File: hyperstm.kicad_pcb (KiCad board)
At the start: 2 copper layers, 71.5 x 70.1 mm, 28 parts, among them J1 USB_B_Micro, J10 SPI1, J2 DBG_HEADER, J3 Micro_SD_Card_Det, J4 Analog_Header, J5 UART_COMBO, J6 USART1, J7 SPI2, J8 I2C1, J9 I2C4, Q3 FDN340P, SW1 SW_SPST, SW2 SW_SPST, U1 STM32L4R5VITx, U2 MIC5219-3.3, U3 S27KL0641

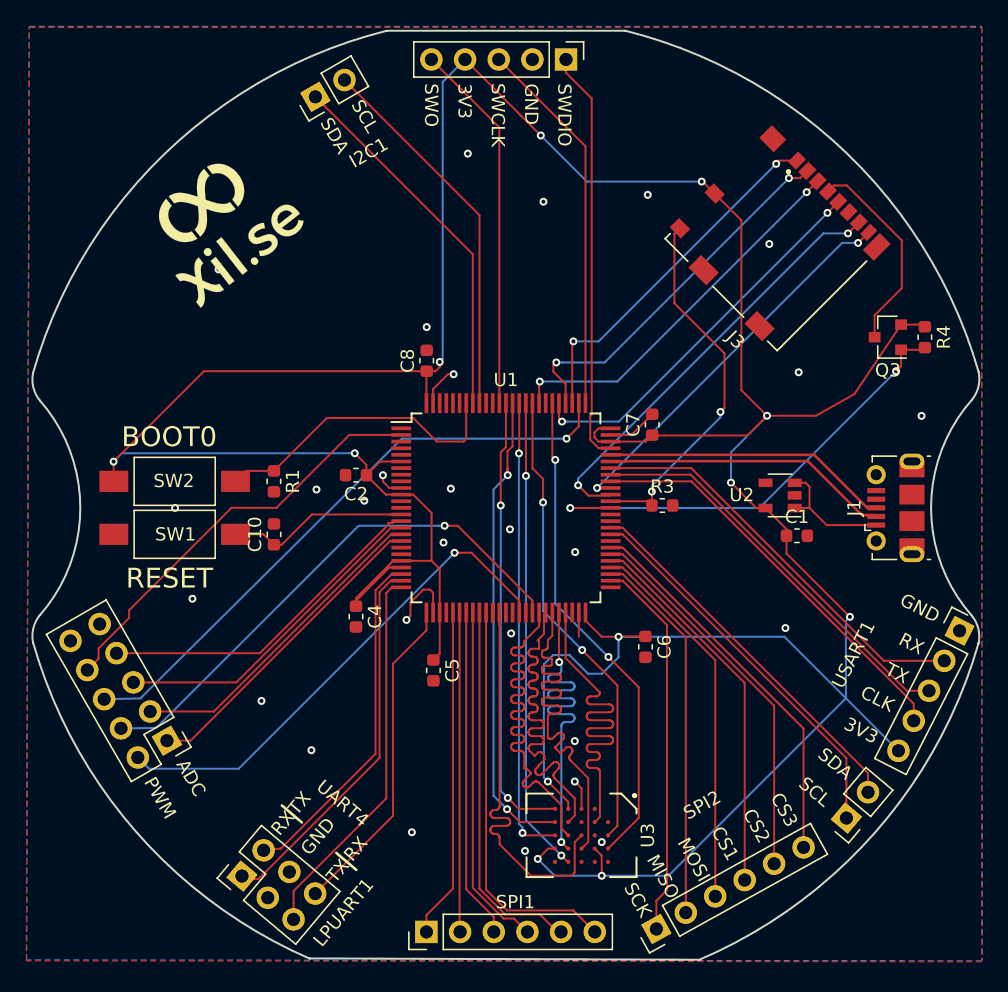
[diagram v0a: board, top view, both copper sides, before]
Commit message: Fix outline
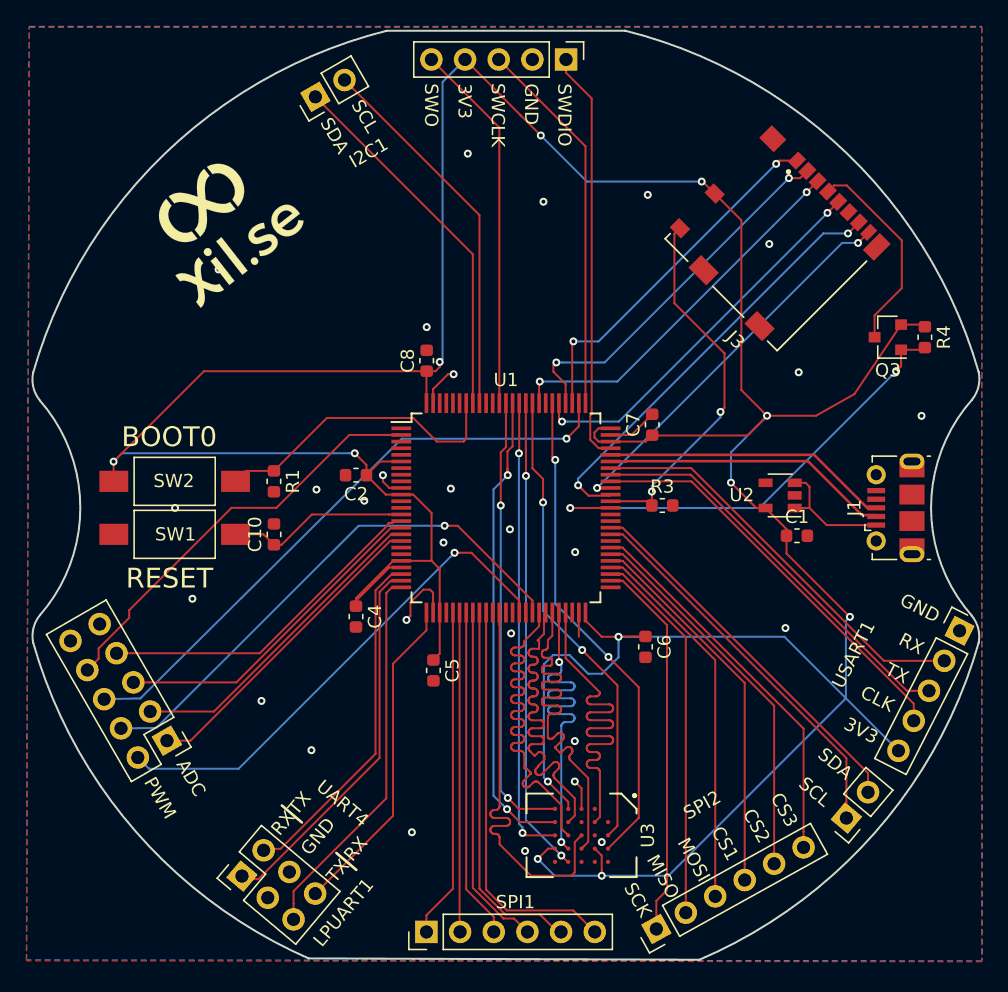
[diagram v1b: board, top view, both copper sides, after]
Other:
- outline, holes or cut-outs redrawn
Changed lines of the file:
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@@
-(kicad_pcb (version 20171130) (host pcbnew 5.0.0-fee4fd1~66~ubuntu18.04.1)
+(kicad_pcb (version 20171130) (host pcbnew 5.1.5+dfsg1-2build2)
   (general
     (thickness 1.6)
@@
     (zone_45_only no)
     (trace_min 0.1524)
-    (segment_width 0.2)
-    (edge_width 0.15)
     (via_size 0.6)
     (via_drill 0.3)
@@
     (uvia_min_size 0.2)
     (uvia_min_drill 0.1)
+    (edge_width 0.15)
+    (segment_width 0.2)
     (pcb_text_width 0.3)
     (pcb_text_size 1.5 1.5)
@@
       (xy 0.186687 3.496485) (xy 0.239391 3.49077) (xy 0.268318 3.491476)) (layer F.SilkS) (width 0.01))
   )
+  (gr_arc (start 183.24 109.71) (end 185.667211 110.189202) (angle -50.74504922) (layer Edge.Cuts) (width 0.15))
+  (gr_arc (start 150.01 100.02) (end 114.322718 110.169442) (angle -50.44715247) (layer Edge.Cuts) (width 0.15))
+  (gr_arc (start 116.75 90.32) (end 114.325521 89.785729) (angle -52.22555031) (layer Edge.Cuts) (width 0.15))
+  (gr_arc (start 116.76 109.67) (end 114.830001 108.100001) (angle -50.7079909) (layer Edge.Cuts) (width 0.15))
   (gr_text PWM (at 123.06 120.43 300) (layer F.SilkS)
     (effects (font (size 1 1) (thickness 0.15)) (justify left))
@@
     (effects (font (size 1.5 1.5) (thickness 0.3)))
   )
-  (gr_arc (start 183.23203 109.71009) (end 185.662029 110.230089) (angle -51.56151773) (layer Edge.Cuts) (width 0.15))
   (gr_arc (start 183.240001 90.269999) (end 185.67 89.75) (angle 51.56151773) (layer Edge.Cuts) (width 0.15))
-  (gr_arc (start 116.749999 109.670001) (end 114.32 110.19) (angle 51.56151773) (layer Edge.Cuts) (width 0.15))
-  (gr_arc (start 116.749999 90.319999) (end 114.32 89.8) (angle -51.56151773) (layer Edge.Cuts) (width 0.15))
   (gr_arc (start 194.386531 99.996635) (end 185.16 91.85) (angle -82.81331583) (layer Edge.Cuts) (width 0.15))
   (gr_arc (start 105.6 100) (end 114.83 108.1) (angle -82.46843144) (layer Edge.Cuts) (width 0.15))
   (gr_arc (start 150 100) (end 185.67 89.75) (angle -59.93141119) (layer Edge.Cuts) (width 0.15))
   (gr_arc (start 150 100) (end 141.000001 64.000001) (angle -59.9863478) (layer Edge.Cuts) (width 0.15))
-  (gr_line (start 141 64) (end 159 64) (layer Edge.Cuts) (width 0.15))
+  (gr_line (start 141.000001 64.000001) (end 159.001348 63.994624) (layer Edge.Cuts) (width 0.15))
   (gr_arc (start 150 100) (end 164.599999 134.099999) (angle -50.87841841) (layer Edge.Cuts) (width 0.15))
-  (gr_arc (start 150 100) (end 114.32 110.17) (angle -50.56745301) (layer Edge.Cuts) (width 0.15))
-  (gr_line (start 135.2 134) (end 164.6 134.1) (layer Edge.Cuts) (width 0.15))
+  (gr_line (start 135.110309 133.999295) (end 164.599999 134.099999) (layer Edge.Cuts) (width 0.15))
   (via (at 155.194 120.65) (size 0.6) (drill 0.3) (layers F.Cu B.Cu) (net 1))
   (segment (start 155.5 109.73) (end 155.5 107.9) (width 0.1524) (layer F.Cu) (net 1))
